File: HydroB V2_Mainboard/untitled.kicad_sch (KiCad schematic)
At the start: 12 parts, among them J3 PH SENSOR, J4 EC SENSOR, U2 SN65HVD72DR

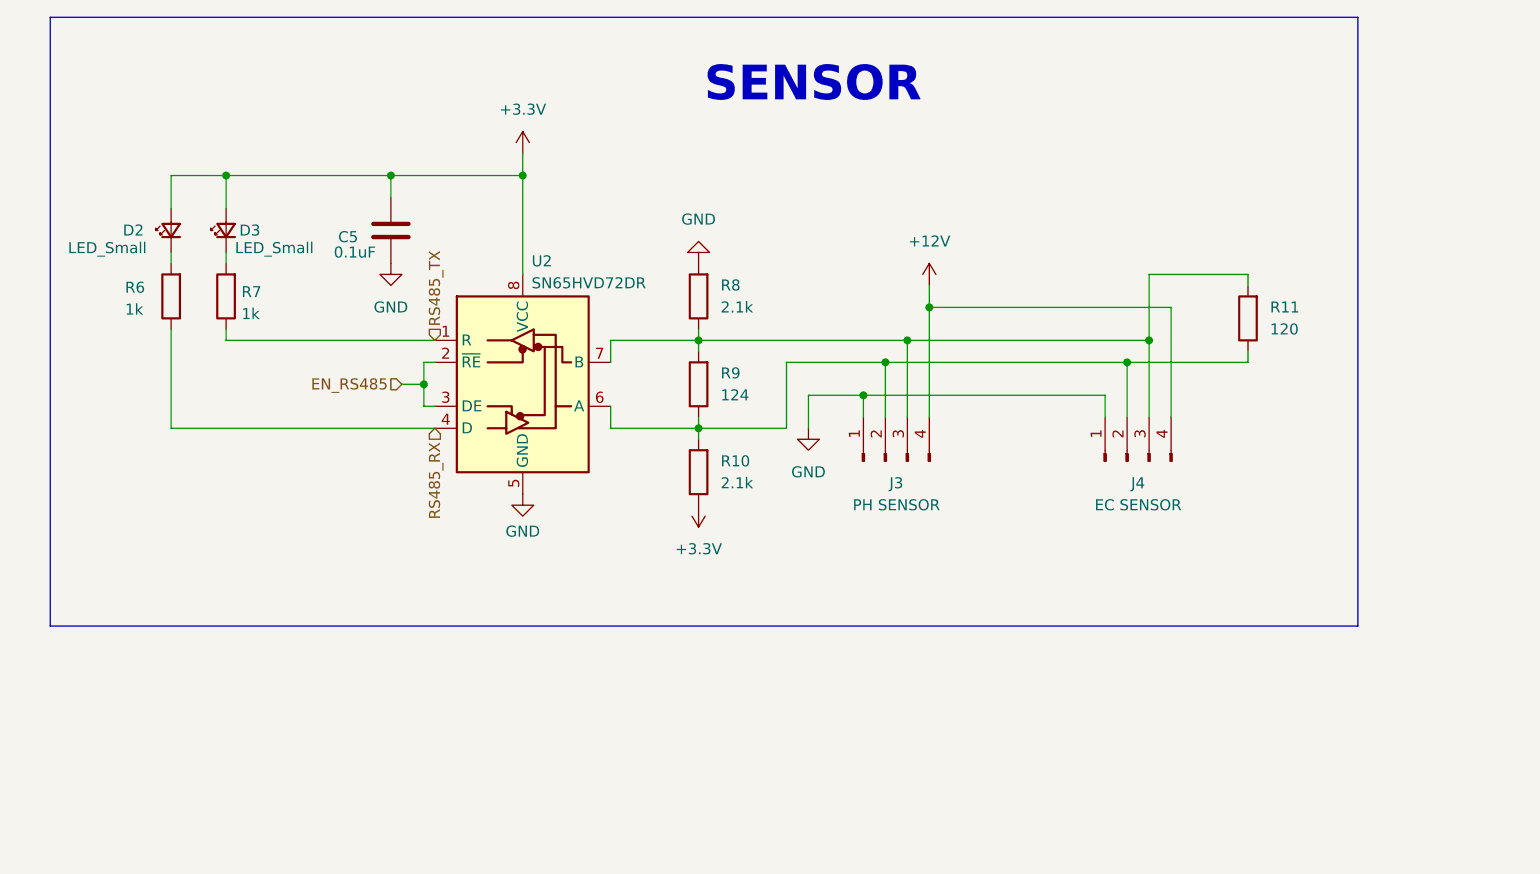
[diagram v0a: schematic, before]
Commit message: Mainboard schematic update
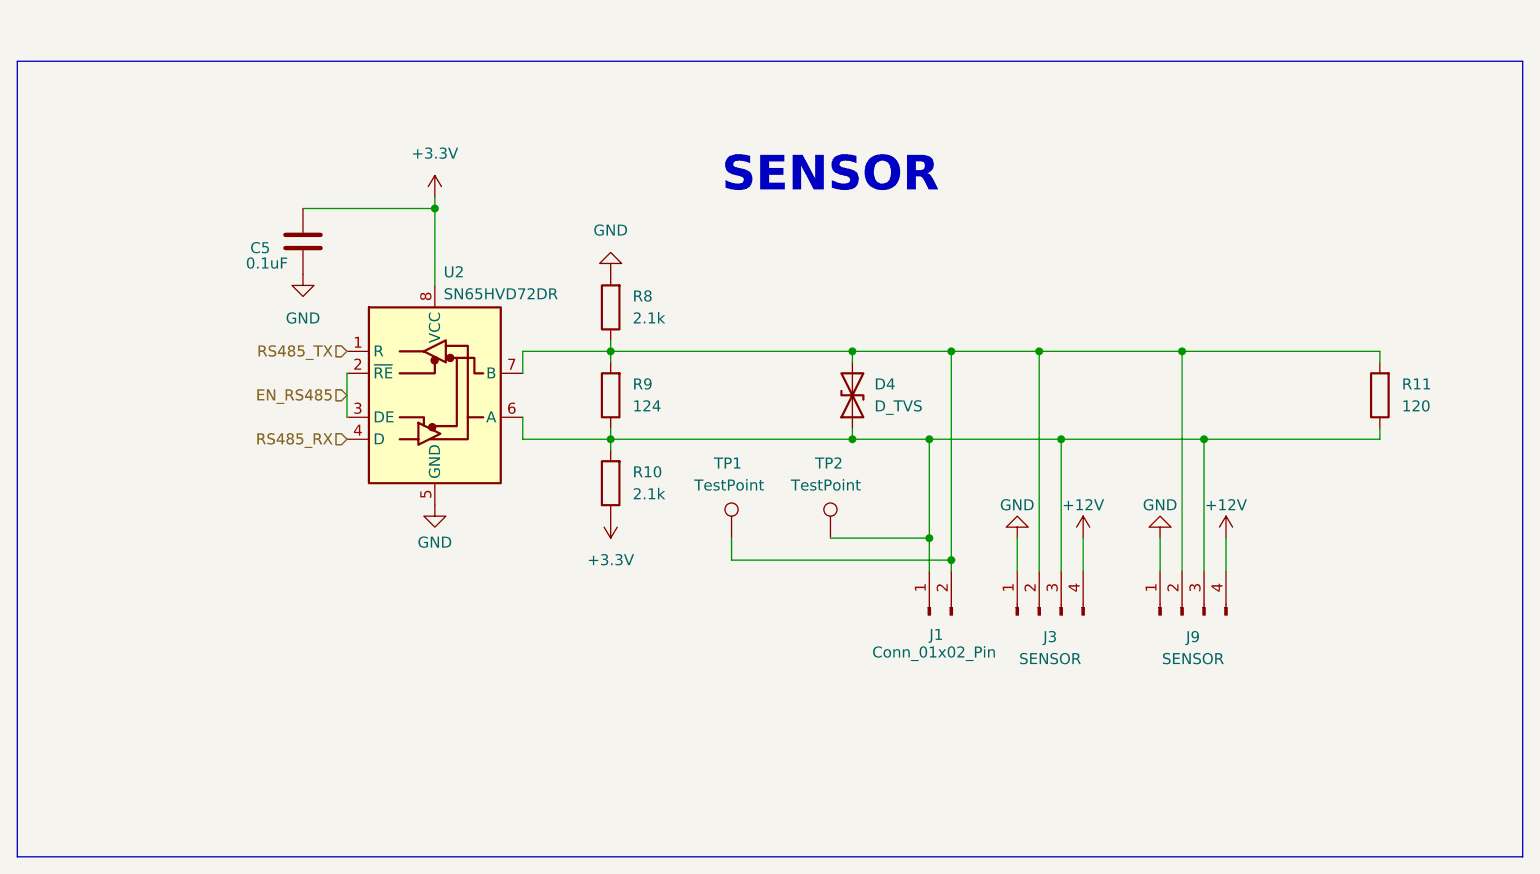
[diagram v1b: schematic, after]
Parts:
- removed D2, D3: LED_Small, LED_SMD:LED_0805_2012Metric, symbol Device:LED_Small
- removed J4: EC SENSOR, Connector_Phoenix_MC:PhoenixContact_MCV_1,5_4-G-3.81_1x04_P3.81mm_Vertical, symbol Connector:Conn_01x04_Pin
- removed R6, R7: 1k, Resistor_SMD:R_0603_1608Metric, symbol Device:R
- added D4: D_TVS, Diode_SMD:D_SOD-123F, symbol Device:D_TVS
- added J1: Conn_01x02_Pin, DC Conn:Modbus, symbol Connector:Conn_01x02_Pin
- added J9: SENSOR, DC Conn:Modbus, symbol Connector:Conn_01x04_Pin
- added TP1, TP2: TestPoint, TestPoint:TestPoint_Loop_D1.80mm_Drill1.0mm_Beaded, symbol Connector:TestPoint
- J3: value PH SENSOR -> SENSOR; footprint Connector_Phoenix_MC:PhoenixContact_MCV_1,5_4-G-3.81_1x04_P3.81mm_Vertical -> DC Conn:Modbus
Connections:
- net +12V: now also J9.4 (Pin_4)
- net GND: now also J9.1 (Pin_1)
- net at R10.2, R11.1, R9.1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: now also J3.3 (Pin_3), D4.1 (A1), J1.1 (Pin_1), J9.3 (Pin_3), TP2.1; no longer J3.2 (Pin_2)
- net at R11.2, R8.1, R9.2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: now also J3.2 (Pin_2), D4.2 (A2), J1.2 (Pin_2), J9.2 (Pin_2), TP1.1; no longer J3.3 (Pin_3)
